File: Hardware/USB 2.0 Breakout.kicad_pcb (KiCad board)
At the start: 2 copper layers, 26 x 20.5 mm, 5 parts, among them J1 Conn_01x04, P1 USB_C_Plug_USB2.0

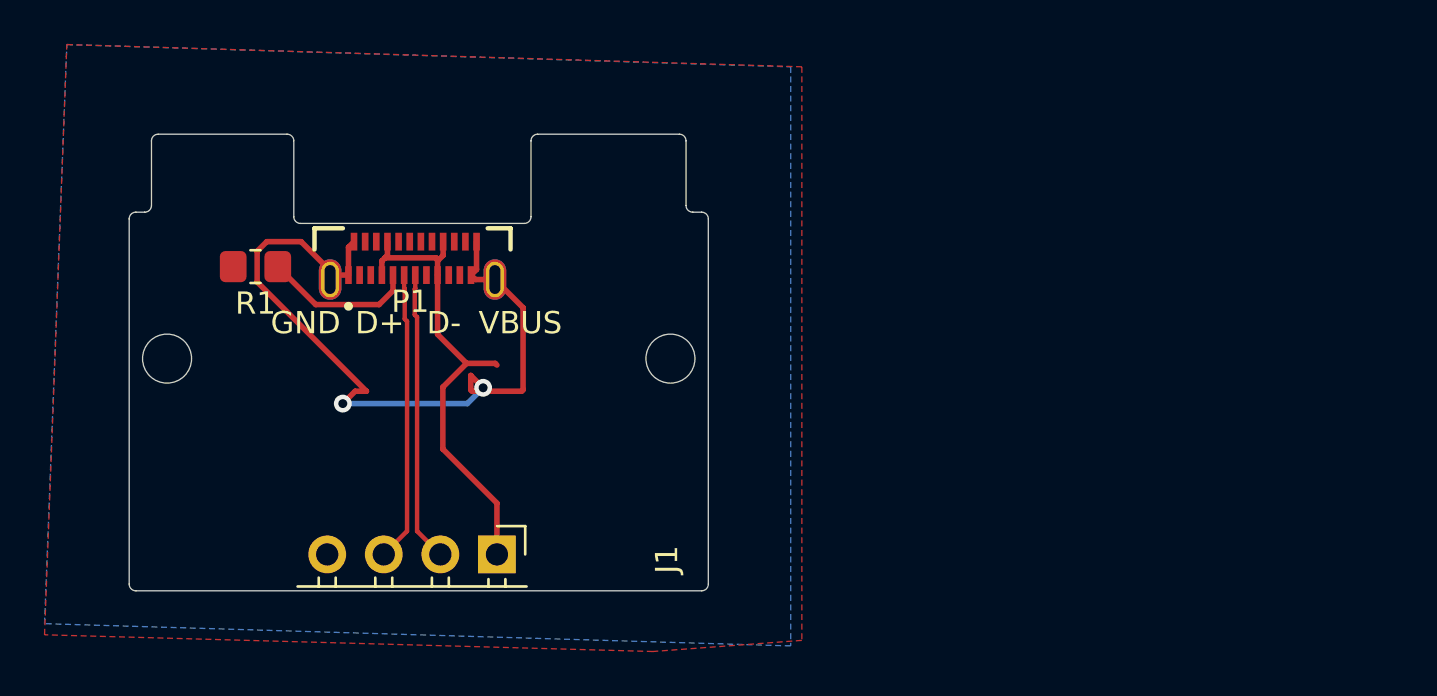
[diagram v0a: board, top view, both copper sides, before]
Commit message: Updated files
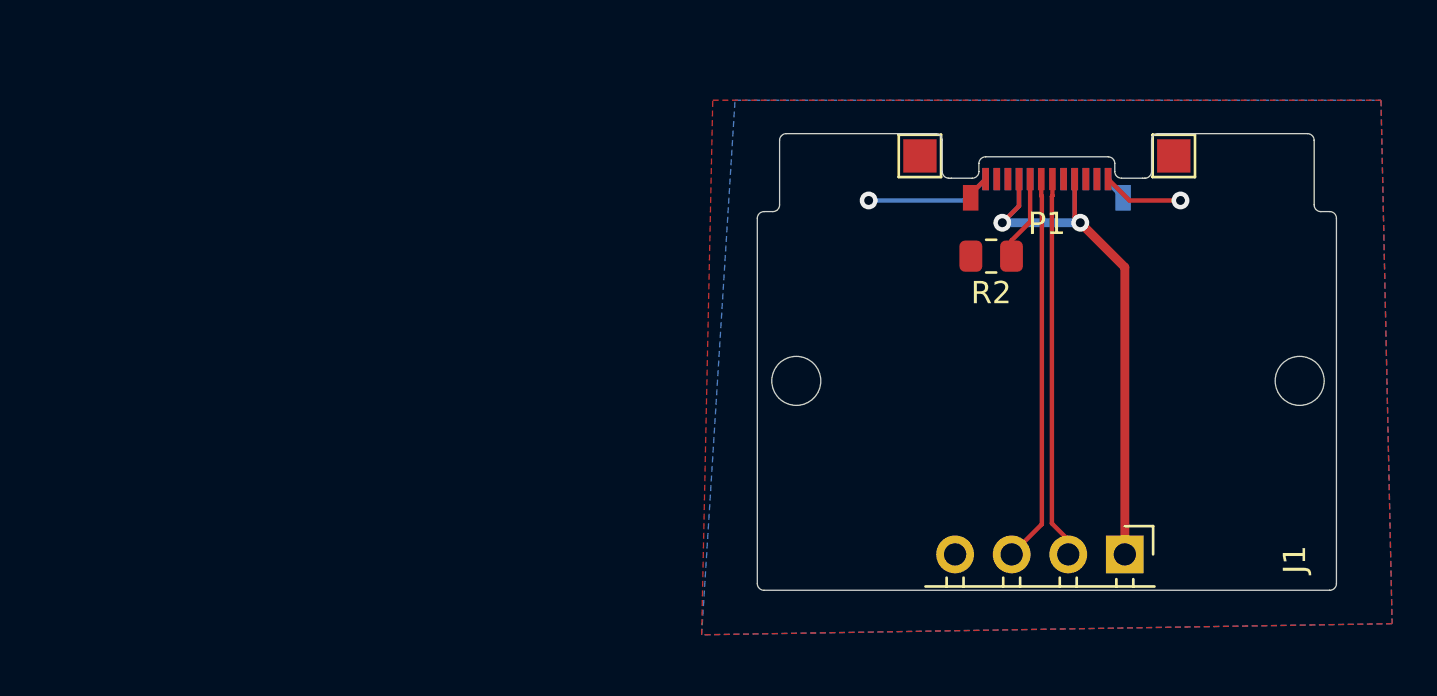
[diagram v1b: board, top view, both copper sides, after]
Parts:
- removed R1: 5.1k Pull-down, Resistor_SMD:R_0805_2012Metric_Pad1.20x1.40mm_HandSolder
- added R2: 5.1k Pull-down, Resistor_SMD:R_0805_2012Metric, F.Cu at (200.5, 65.0)
- added TP1: TestPoint, TestPoint:TestPoint_Pad_1.5x1.5mm, F.Cu at (197.3, 60.5)
- added TP3: TestPoint, TestPoint:TestPoint_Pad_1.5x1.5mm, F.Cu at (208.7, 60.5)
- P1: footprint SnapEDA Library:GCT_USB4155-03-C_REVA -> Expansion_Card:USB_C_Plug_Molex_105444
- moved P1 28.7 mm to (203.0, 61.5), turned to 0 degrees
- moved H1 28.3 mm to (191.8, 70.6)
- moved H2 28.3 mm to (214.3, 70.6)
- moved J1 28.2 mm to (206.5, 78.4)
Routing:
- net Earth: track 35.8 -> 11.5 mm
- net VBUS: track 21.6 -> 27.9 mm, vias 0 -> 2
- net D+: track 13.0 -> 17.4 mm
- net D-: track 13.0 -> 17.2 mm
- net CC: track 6.84 -> 3.81 mm
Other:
- outline, holes or cut-outs redrawn
- board text removed: "D+"
- board text removed: "D-"
- board text removed: "GND"
- board text removed: "VBUS"
